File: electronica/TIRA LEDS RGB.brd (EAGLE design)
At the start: 160 x 100 mm, 6 parts

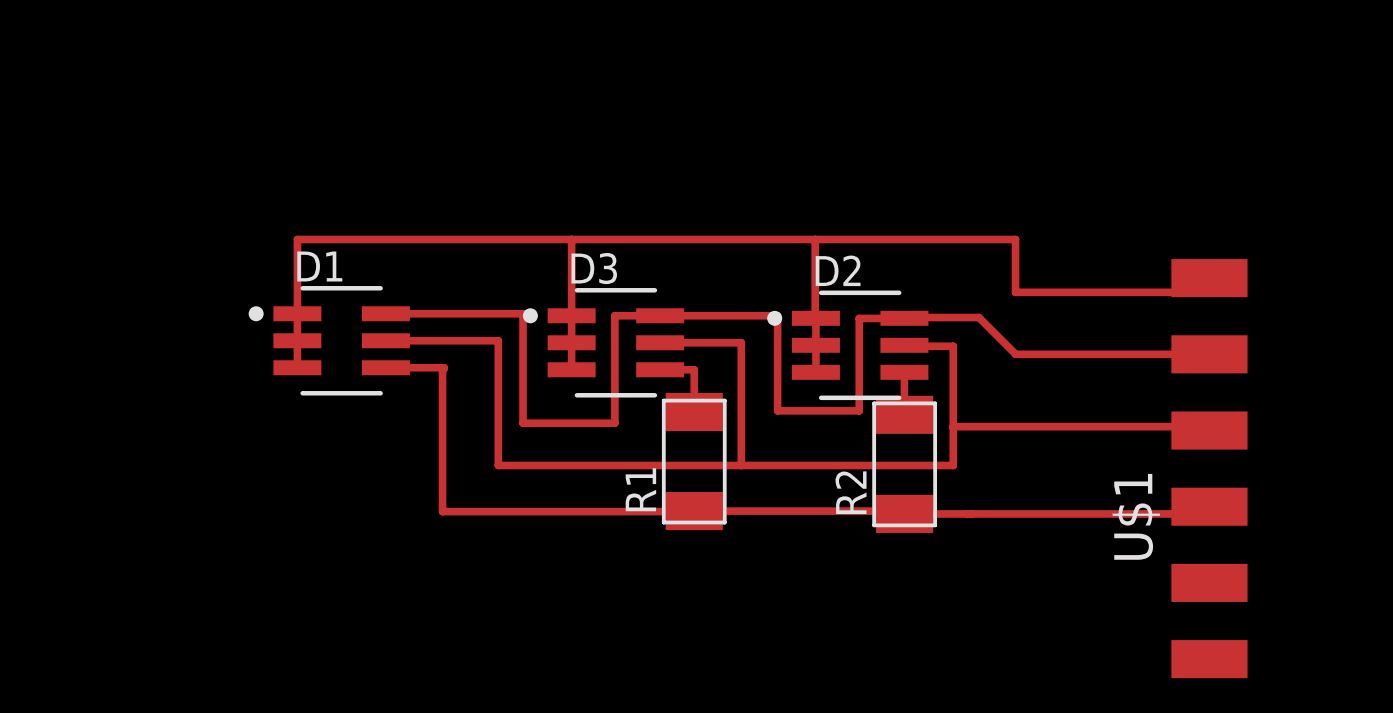
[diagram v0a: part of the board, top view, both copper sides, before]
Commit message: Add files via upload
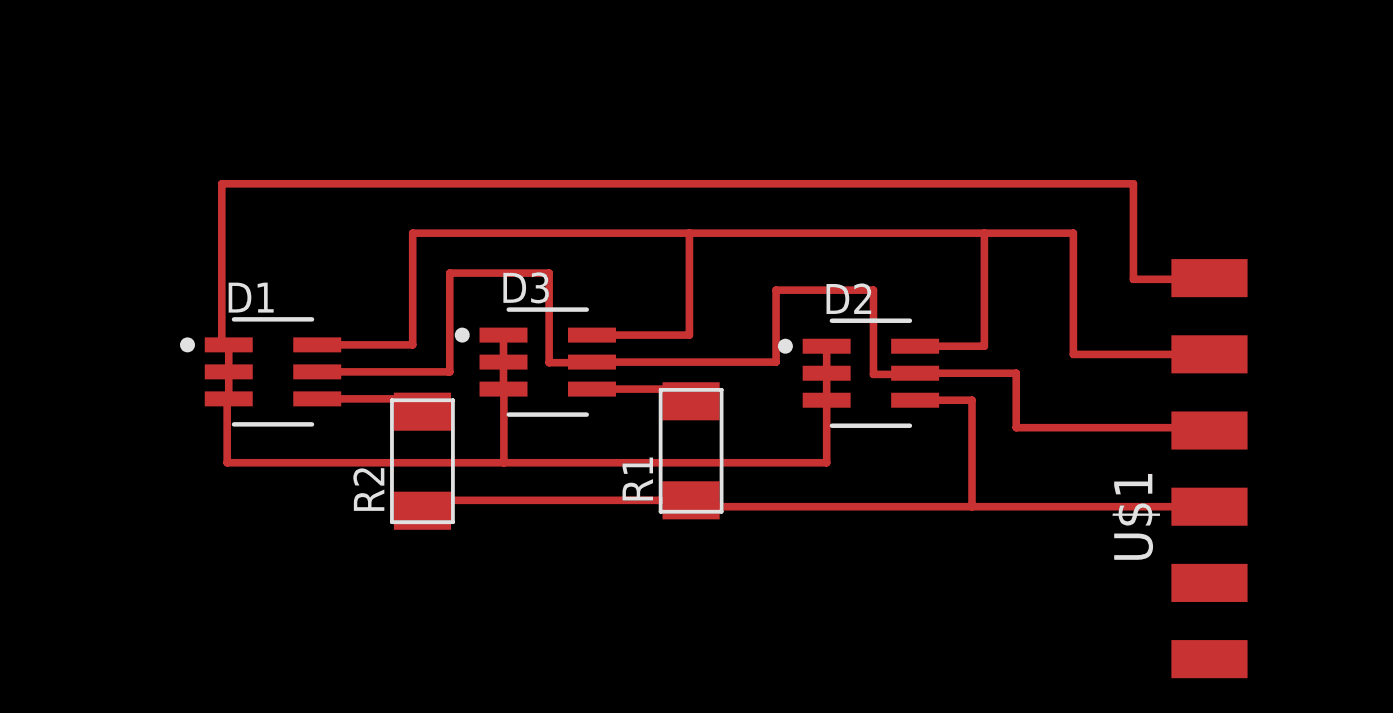
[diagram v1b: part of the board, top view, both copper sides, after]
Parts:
- moved R2 16.1 mm to (40.0, 34.2)
- moved D1 2.51 mm to (35.1, 37.1)
- moved D3 2.36 mm to (44.2, 37.5)
- moved D2 1.00 mm to (55.0, 37.1)
- moved R1 0.37 mm to (49.0, 34.5)
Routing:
- net VCC: track 45.2 -> 73.9 mm
- net BLUE: track 41.5 -> 50.3 mm
- net RED: track 36.9 -> 42.1 mm
- net GREEN: track 44.3 -> 43.4 mm
